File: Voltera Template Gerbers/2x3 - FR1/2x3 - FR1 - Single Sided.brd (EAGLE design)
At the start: 135 x 101.6 mm, 1 part

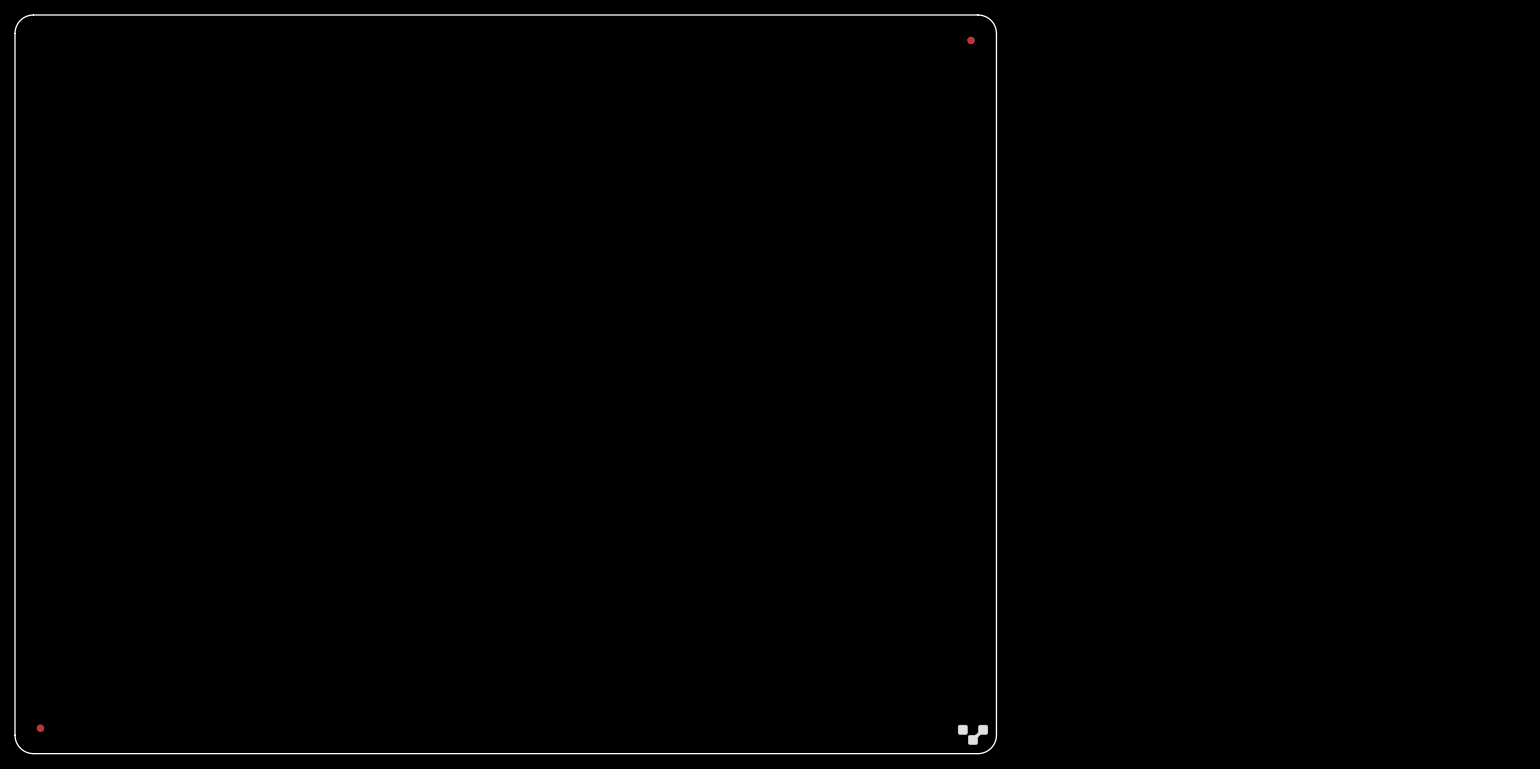
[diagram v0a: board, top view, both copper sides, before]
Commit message: Created FAB version for evertying, removed bad versions
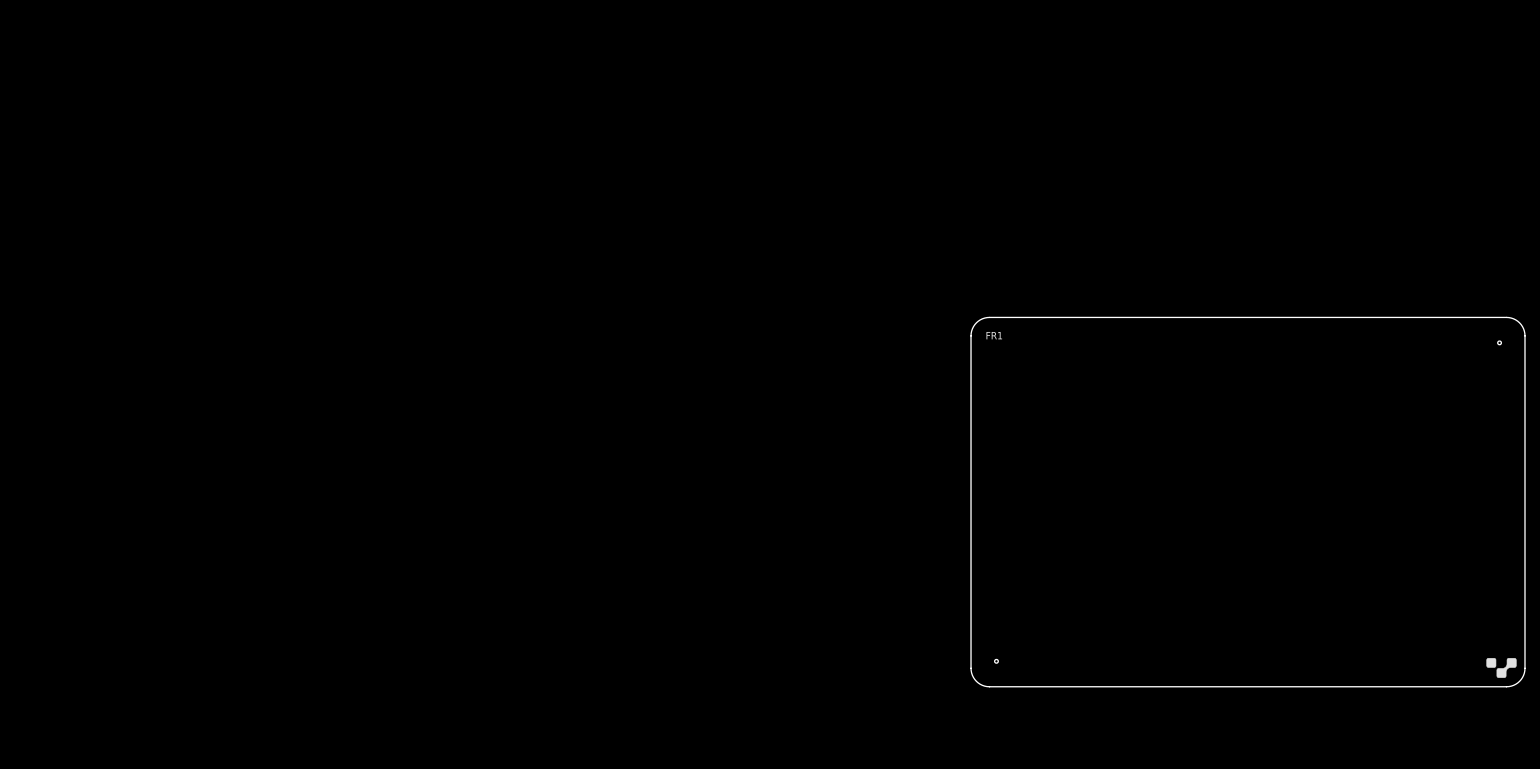
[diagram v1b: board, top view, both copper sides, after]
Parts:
- E$1: device voltera_EAGLE_community_lib:4X5_BOARD -> voltera_EAGLE_community_lib:2X3_BOARD_FR1_RAW
- moved E$1 131.8 mm to (0.00, 0.00)
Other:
- board size 135 x 101.6 mm -> 76.2 x 50.8 mm
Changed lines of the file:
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@@
 <?xml version="1.0" encoding="utf-8"?>
 <!DOCTYPE eagle SYSTEM "eagle.dtd">
-<eagle version="8.7.0">
+<eagle version="8.7.1">
 <drawing>
 <settings>
@@
 <layer number="27" name="tValues" color="7" fill="1" visible="yes" active="yes"/>
 <layer number="28" name="bValues" color="7" fill="1" visible="yes" active="yes"/>
-<layer number="29" name="tStop" color="7" fill="3" visible="no" active="yes"/>
-<layer number="30" name="bStop" color="7" fill="6" visible="no" active="yes"/>
-<layer number="31" name="tCream" color="7" fill="4" visible="no" active="yes"/>
-<layer number="32" name="bCream" color="7" fill="5" visible="no" active="yes"/>
-<layer number="33" name="tFinish" color="6" fill="3" visible="no" active="yes"/>
-<layer number="34" name="bFinish" color="6" fill="6" visible="no" active="yes"/>
-<layer number="35" name="tGlue" color="7" fill="4" visible="no" active="yes"/>
-<layer number="36" name="bGlue" color="7" fill="5" visible="no" active="yes"/>
-<layer number="37" name="tTest" color="7" fill="1" visible="no" active="yes"/>
-<layer number="38" name="bTest" color="7" fill="1" visible="no" active="yes"/>
+<layer number="29" name="tStop" color="7" fill="3" visible="yes" active="yes"/>
+<layer number="30" name="bStop" color="7" fill="6" visible="yes" active="yes"/>
+<layer number="31" name="tCream" color="7" fill="4" visible="yes" active="yes"/>
+<layer number="32" name="bCream" color="7" fill="5" visible="yes" active="yes"/>
+<layer number="33" name="tFinish" color="6" fill="3" visible="yes" active="yes"/>
+<layer number="34" name="bFinish" color="6" fill="6" visible="yes" active="yes"/>
+<layer number="35" name="tGlue" color="7" fill="4" visible="yes" active="yes"/>
+<layer number="36" name="bGlue" color="7" fill="5" visible="yes" active="yes"/>
+<layer number="37" name="tTest" color="7" fill="1" visible="yes" active="yes"/>
+<layer number="38" name="bTest" color="7" fill="1" visible="yes" active="yes"/>
 <layer number="39" name="tKeepout" color="4" fill="11" visible="yes" active="yes"/>
 <layer number="40" name="bKeepout" color="1" fill="11" visible="yes" active="yes"/>
@@
 <layer number="42" name="bRestrict" color="1" fill="10" visible="yes" active="yes"/>
 <layer number="43" name="vRestrict" color="2" fill="10" visible="yes" active="yes"/>
-<layer number="44" name="Drills" color="7" fill="1" visible="no" active="yes"/>
-<layer number="45" name="Holes" color="7" fill="1" visible="no" active="yes"/>
-<layer number="46" name="Milling" color="3" fill="1" visible="no" active="yes"/>
+<layer number="44" name="Drills" color="7" fill="1" visible="yes" active="yes"/>
+<layer number="45" name="Holes" color="7" fill="1" visible="yes" active="yes"/>
+<layer number="46" name="Milling" color="3" fill="1" visible="yes" active="yes"/>
 <layer number="47" name="Measures" color="7" fill="1" visible="yes" active="yes"/>
 <layer number="48" name="Document" color="7" fill="1" visible="yes" active="yes"/>
@@
 <layer number="112" name="tSilk" color="7" fill="1" visible="yes" active="yes"/>
 <layer number="113" name="IDFDebug" color="4" fill="1" visible="yes" active="yes"/>
+<layer number="114" name="Badge_Outline" color="7" fill="1" visible="yes" active="yes"/>
+<layer number="115" name="ReferenceISLANDS" color="7" fill="1" visible="yes" active="yes"/>
 <layer number="116" name="Patch_BOT" color="9" fill="4" visible="yes" active="yes"/>
 <layer number="118" name="Rect_Pads" color="7" fill="1" visible="no" active="no"/>
@@
 <layer number="223" name="223bmp" color="24" fill="1" visible="no" active="no"/>
 <layer number="224" name="224bmp" color="25" fill="1" visible="no" active="no"/>
+<layer number="225" name="225bmp" color="7" fill="1" visible="yes" active="yes"/>
+<layer number="226" name="226bmp" color="7" fill="1" visible="yes" active="yes"/>
+<layer number="227" name="227bmp" color="7" fill="1" visible="yes" active="yes"/>
+<layer number="228" name="228bmp" color="7" fill="1" visible="yes" active="yes"/>
+<layer number="229" name="229bmp" color="7" fill="1" visible="yes" active="yes"/>
+<layer number="230" name="230bmp" color="7" fill="1" visible="yes" active="yes"/>
 <layer number="231" name="Eagle3D_PG1" color="7" fill="1" visible="no" active="no"/>
 <layer number="232" name="Eagle3D_PG2" color="7" fill="1" visible="no" active="no"/>
@@
 <layer number="251" name="SMDround" color="12" fill="11" visible="no" active="no"/>
 <layer number="254" name="cooling" color="7" fill="1" visible="yes" active="yes"/>
+<layer number="255" name="routoute" color="7" fill="1" visible="yes" active="yes"/>
 </layers>
 <board>
@@
 </autorouter>
 <elements>
-<element name="E$1" library="voltera_EAGLE_community_lib" package="4X5_BOARD" value="" x="-131.5" y="-9.2"/>
+<element name="E$1" library="voltera_EAGLE_community_lib" package="2X3_BOARD_FR1_RAW" value="" x="0" y="0"/>
 </elements>
 <signals>
